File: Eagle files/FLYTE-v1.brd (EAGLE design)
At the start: 116 x 55 mm, 49 parts, among them J2 CONSMA002, Q1 IRF540NPBF, Q2 IRF540NPBF, SW1 1825159-1, U3 CORE1262-868M, U6 W25Q32JVSSIQ

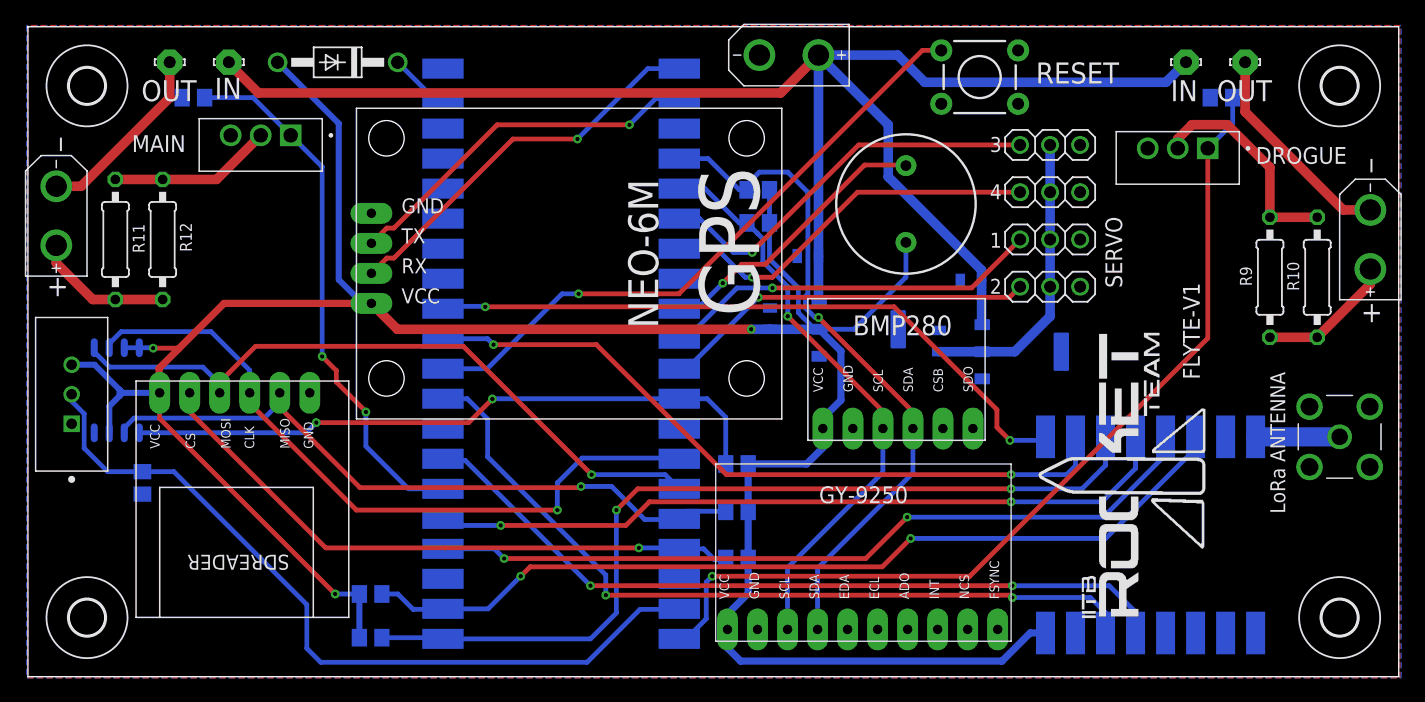
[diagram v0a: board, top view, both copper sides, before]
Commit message: Minor fixes
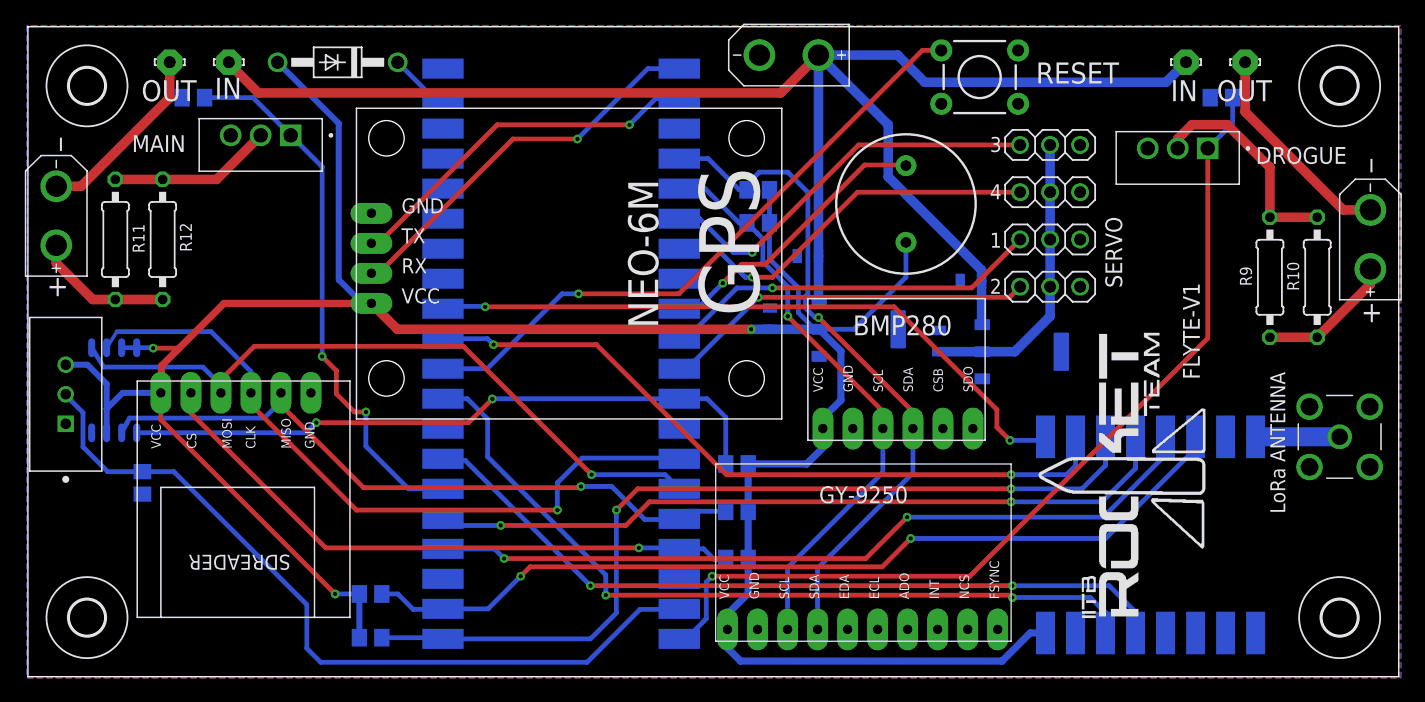
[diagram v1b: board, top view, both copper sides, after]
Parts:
- moved SW1 0.50 mm to (3.20, 23.9)
- moved U6 0.22 mm to (7.30, 24.2)
- moved U$3 0.10 mm to (9.25, 25.0)
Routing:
- net 3V3: track 220.5 -> 221.2 mm
- net MAIN: track 45.6 -> 46.1 mm
